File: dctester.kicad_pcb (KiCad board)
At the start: 2 copper layers, 1 part

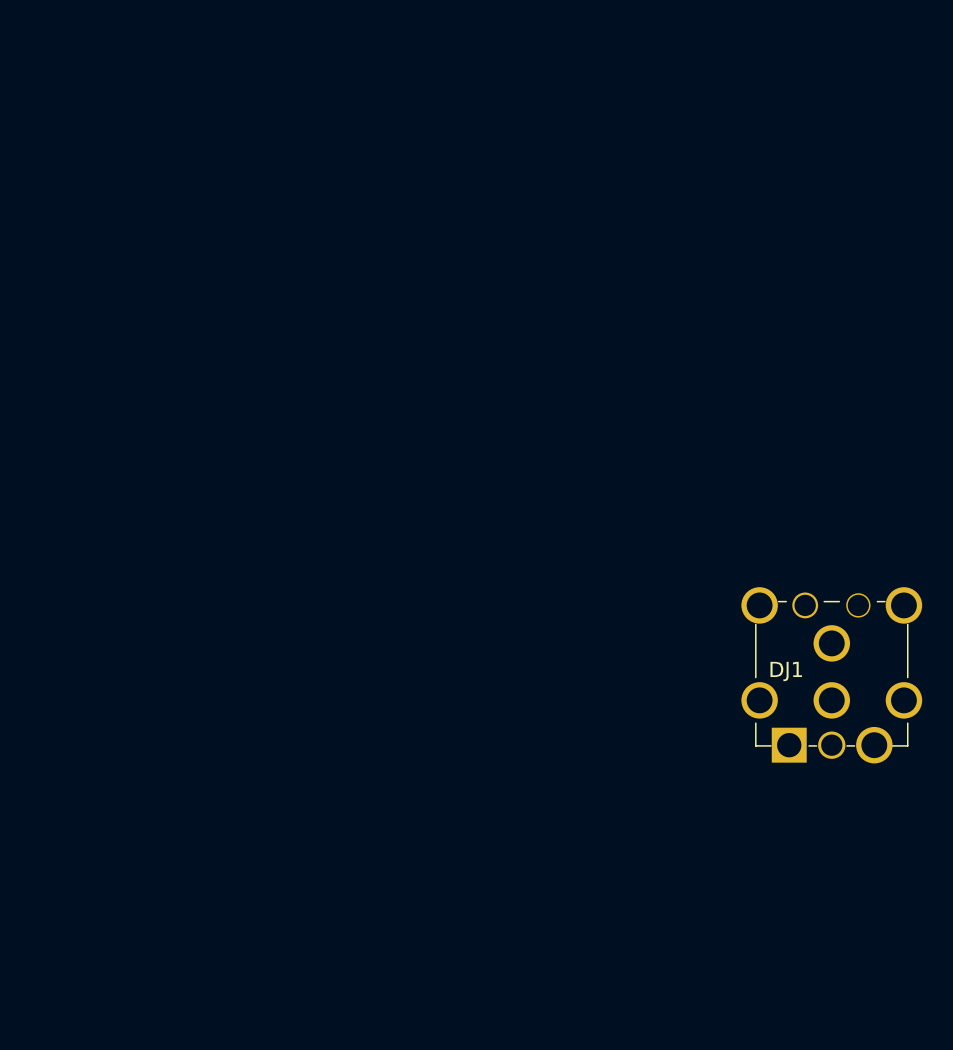
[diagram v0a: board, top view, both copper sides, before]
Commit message: latest
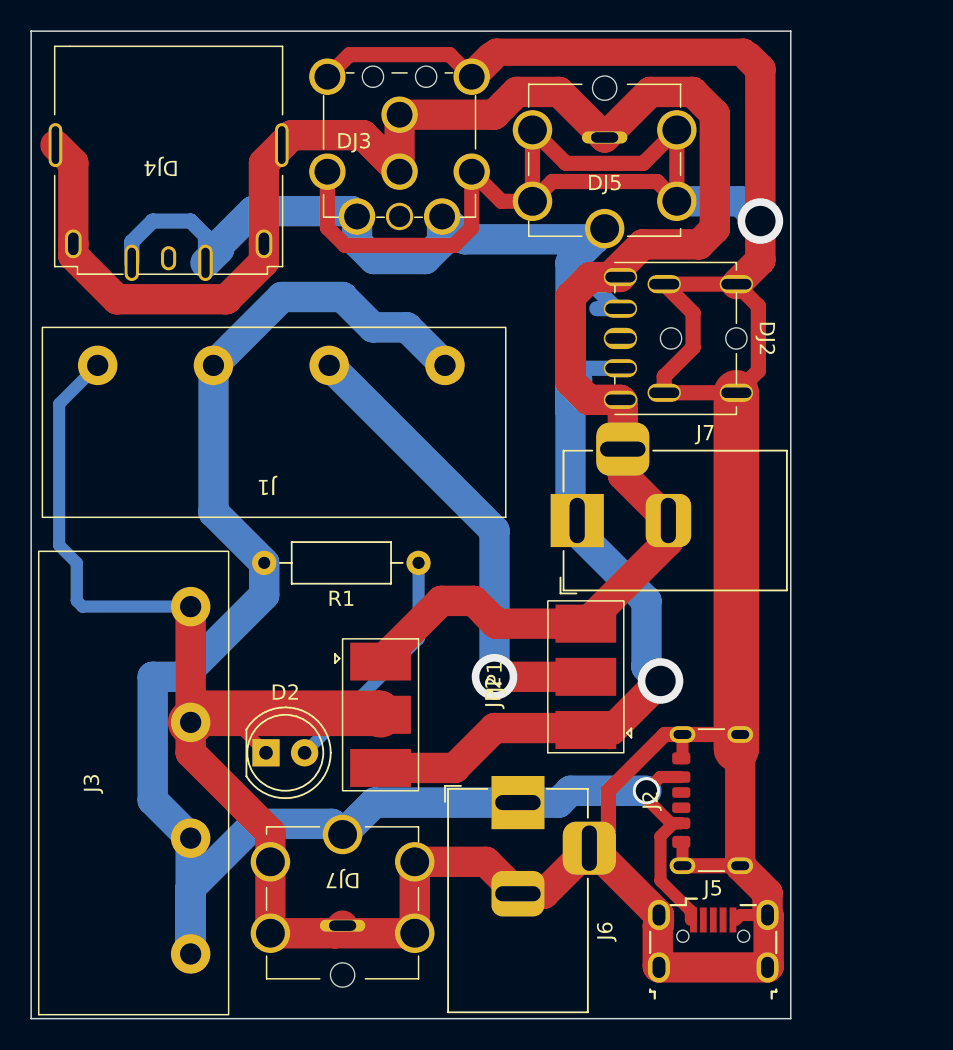
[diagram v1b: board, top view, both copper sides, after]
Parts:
- removed DJ1: ~, mypretties:lenovo_hp_dell_7.4x5mm_dc
- added D2: LED, LED_THT:LED_D5.0mm, F.Cu at (102.5, 107.5)
- added DJ2: HP4.5x3, mypretties:hp_4.5x3.0mm_dc, F.Cu at (133.4, 80.2)
- added DJ3: HP_DELL_LENOVO_7.4x5.5, mypretties:lenovo_hp_dell_7.4x5mm_dc, F.Cu at (111.2, 69.2)
- added DJ4: LENOVO_SQR, mypretties:lenovo_square_dc, F.Cu at (96.0, 74.0)
- added DJ5: DC5.5x2.5, mypretties:general_5.5x2.5mm_dc, F.Cu at (124.8, 61.0)
- added DJ7: DC5.5x2.5, mypretties:general_5.5x2.5mm_dc, F.Cu at (107.5, 124.9)
- added J1: Screw_Terminal_01x04, mypretties:screw762, F.Cu at (114.2, 82.0)
- added J2: USB_C_Receptacle_PowerOnly_6P, mypretties:USB_C_Receptacle_GCT_USB4125-xx-x-0190_6P_TopMnt_Horizontal, F.Cu at (132.9, 110.6)
- added J3: Screw_Terminal_01x04, mypretties:screw762, F.Cu at (97.5, 120.7)
- added J5: USB_B_Micro, mypretties:USB_Micro-B_flat_horizon, F.Cu at (131.9, 118.2)
- added J6: DC5.5x2.1, mypretties:BarrelJack_Horizontal, F.Cu at (119.0, 110.8)
- added J7: DC5.5x2.1, mypretties:BarrelJack_Horizontal, F.Cu at (122.9, 92.2)
- added JP1: SolderJumper_3_Open, mypretties:SolderJumper-3_P4.0mm, F.Cu at (123.5, 102.5)
- added JP2: SolderJumper_3_Open, mypretties:SolderJumper-3_P4.0mm, F.Cu at (110.0, 105.0)
- added R1: 2K, Resistor_THT:R_Axial_DIN0207_L6.3mm_D2.5mm_P10.16mm_Horizontal, F.Cu at (112.5, 95.0)
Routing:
- net GND: track 0.00 -> 308.4 mm, vias 0 -> 1
- net outside: track 0.00 -> 132.3 mm
- net /main/VDD: track 0.00 -> 118.9 mm, vias 0 -> 1
- net inside: track 0.00 -> 111.0 mm, vias 0 -> 1
- net Net-(J1-Pin_2): track 0.00 -> 32.0 mm, vias 0 -> 1
- net Net-(D2-A): track 0.00 -> 15.6 mm
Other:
- board outline added: 50 x 65 mm
